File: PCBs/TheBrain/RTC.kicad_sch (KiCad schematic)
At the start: 14 parts, among them J1 Molex 470531000, U4 PCF85063AT/AAZ, U5 EMC2301-1-ACZL-TR, U6 74LVC1G07SE-7, Y1 X32K768S301

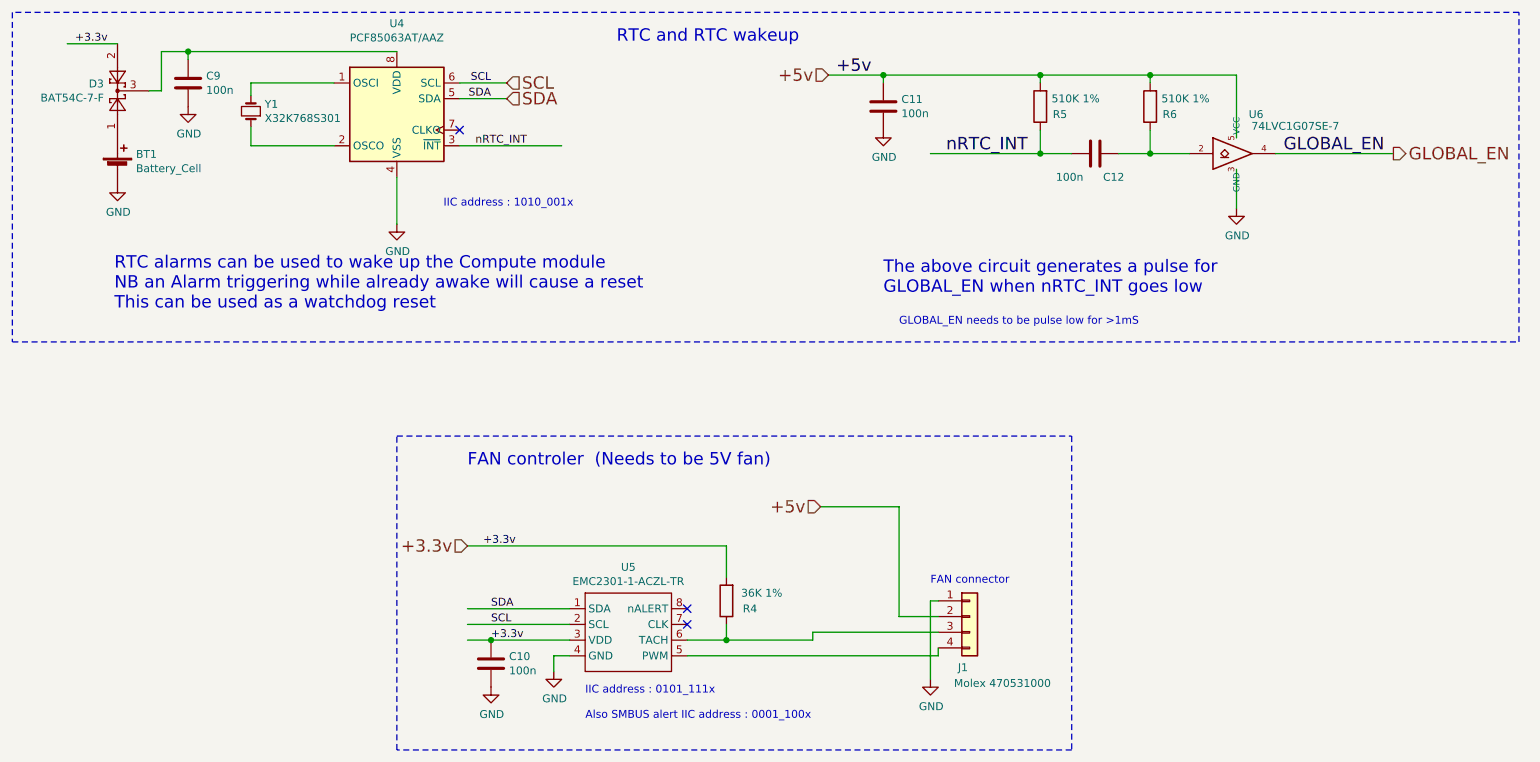
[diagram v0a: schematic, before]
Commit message: Started Brain PCB
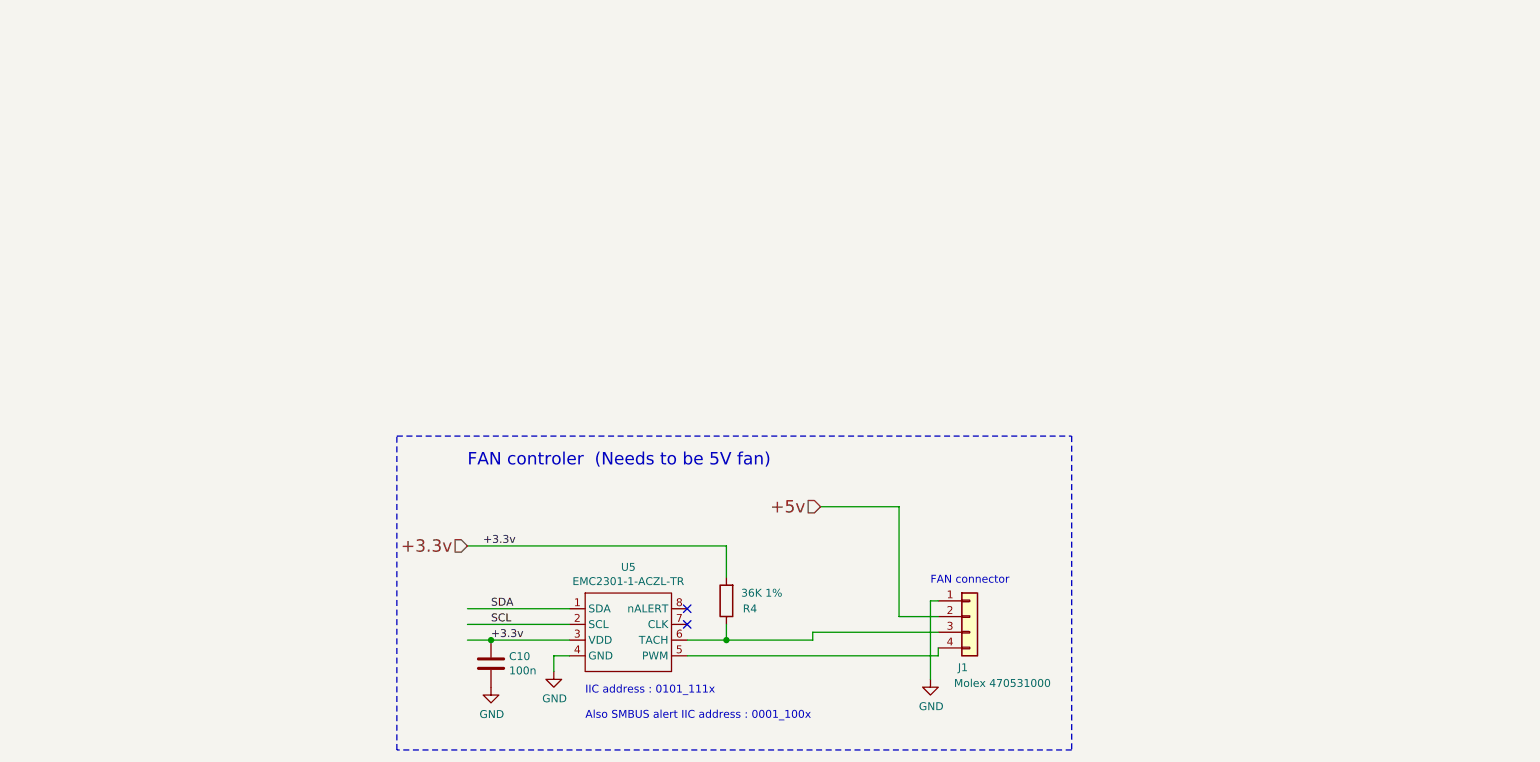
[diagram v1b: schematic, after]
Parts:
- removed BT1: Battery_Cell, Battery:BatteryHolder_Keystone_3034_1x20mm, symbol Device:Battery_Cell
- removed C11, C12, C9: 100n, Capacitor_SMD:C_0402_1005Metric, symbol Device:C
- removed D3: BAT54C-7-F, Package_TO_SOT_SMD:SOT-23, symbol Diode:BAT54C
- removed R5, R6: 510K 1%, Resistor_SMD:R_0402_1005Metric, symbol Device:R
- removed U4: PCF85063AT/AAZ, Package_SO:SOIC-8_3.9x4.9mm_P1.27mm, symbol Timer_RTC:PCF8563T
- removed U6: 74LVC1G07SE-7, Package_TO_SOT_SMD:SOT-353_SC-70-5, symbol CM4IO:74LVC1G07_copy
- removed Y1: X32K768S301, Crystal:Crystal_SMD_3215-2Pin_3.2x1.5mm, symbol Device:Crystal_Small
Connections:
- no-connect marks 3 -> 2
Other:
- note removed: "GLOBAL_EN needs to be pulse low for >1mS"
- note removed: "IIC address : 1010_001x"
- note removed: "RTC alarms can be used to wake up the Compute module NB an Alarm triggering while already awake will cause a reset This can be used as a watchdog reset"
- note removed: "RTC and RTC wakeup"
- note removed: "The above circuit generates a pulse for GLOBAL_EN when nRTC_INT goes low"
